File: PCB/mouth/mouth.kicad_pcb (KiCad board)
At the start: 2 copper layers, 49.6 x 50 mm, 61 parts, among them J1 Screw_Terminal_01x02, J2 Conn_01x04, J3 Conn_01x08, J5 Conn_02x08_Odd_Even, U1 RP2040, U2 W25Q32JVSS, U3 AP2112K-3.3, U4 74AHCT244, U5 74AHCT244, Y1 12MHz

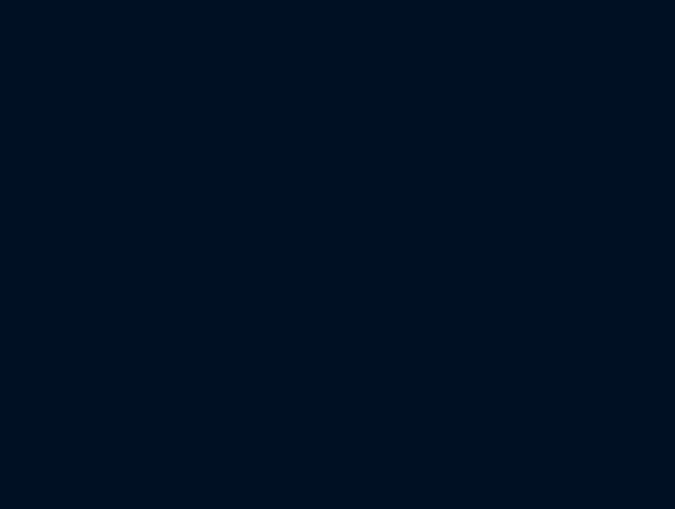
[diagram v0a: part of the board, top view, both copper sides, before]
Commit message: mostly do power part
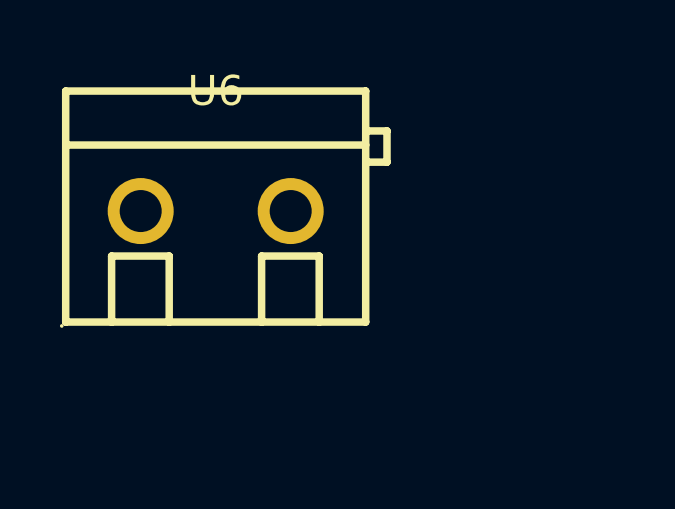
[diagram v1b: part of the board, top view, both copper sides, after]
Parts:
- added U6: KF301-5.0-2P, easyeda2kicad:CONN-TH_P5.00_KF301-5.0-2P, F.Cu at (5.19, 4.12)

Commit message: newBenderCAD
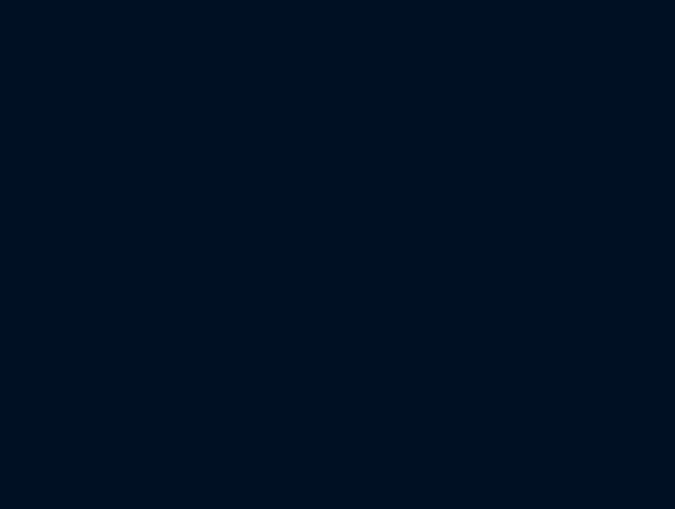
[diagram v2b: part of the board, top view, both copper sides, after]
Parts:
- removed U6: KF301-5.0-2P, easyeda2kicad:CONN-TH_P5.00_KF301-5.0-2P
